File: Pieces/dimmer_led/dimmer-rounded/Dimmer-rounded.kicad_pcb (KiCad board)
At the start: 2 copper layers, 67 x 56 mm, 41 parts, among them J1 Conn_01x02_Female, J2 Conn_01X03, J3 TB_1X2, J4 Conn_01x03_Female, J5 TB_1X2, J6 TB_1X2, Q1 BTA06-600C, Q2 BTA06-600C, Q3 BTA06-600C, Q5 2N7000, U1 LM78XX, U14 LM324, U3 MOC3020M, U4 MOC3020M, U5 MOC3020M, U7 PC817

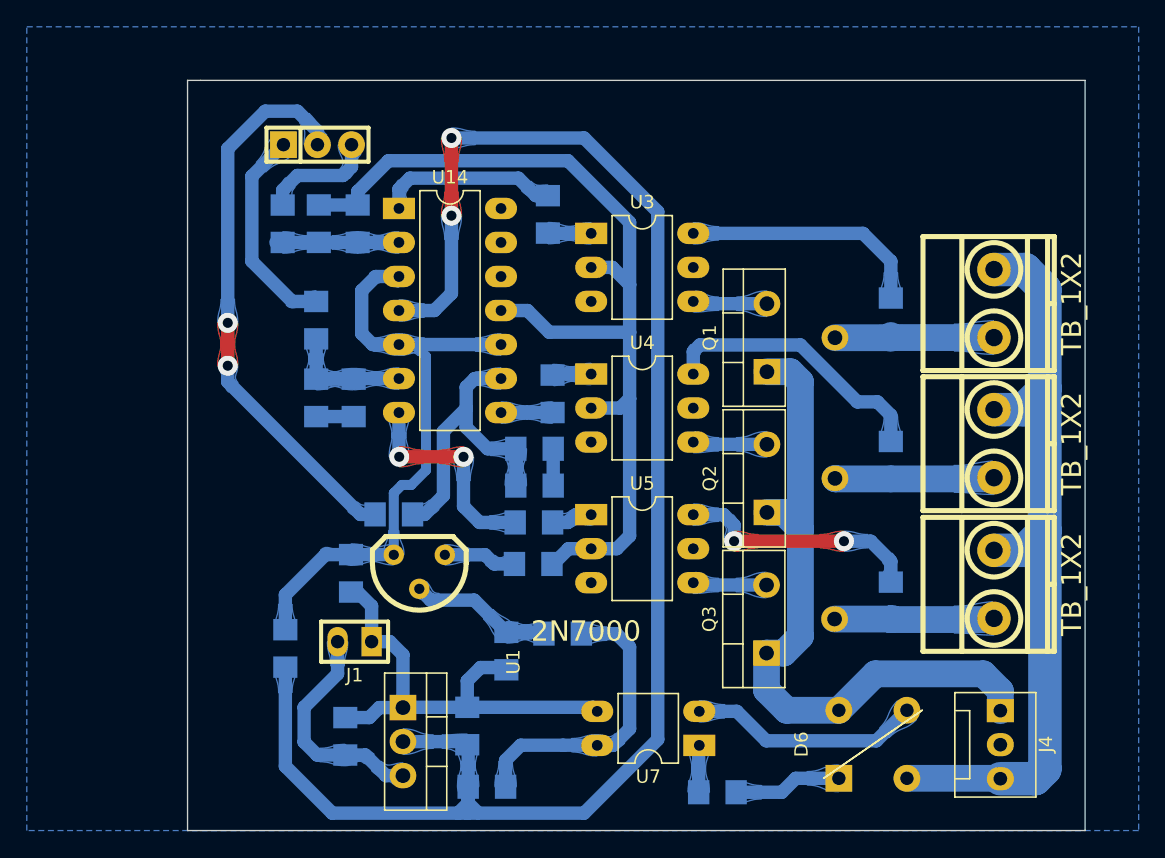
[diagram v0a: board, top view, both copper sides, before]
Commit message: lista de componentes
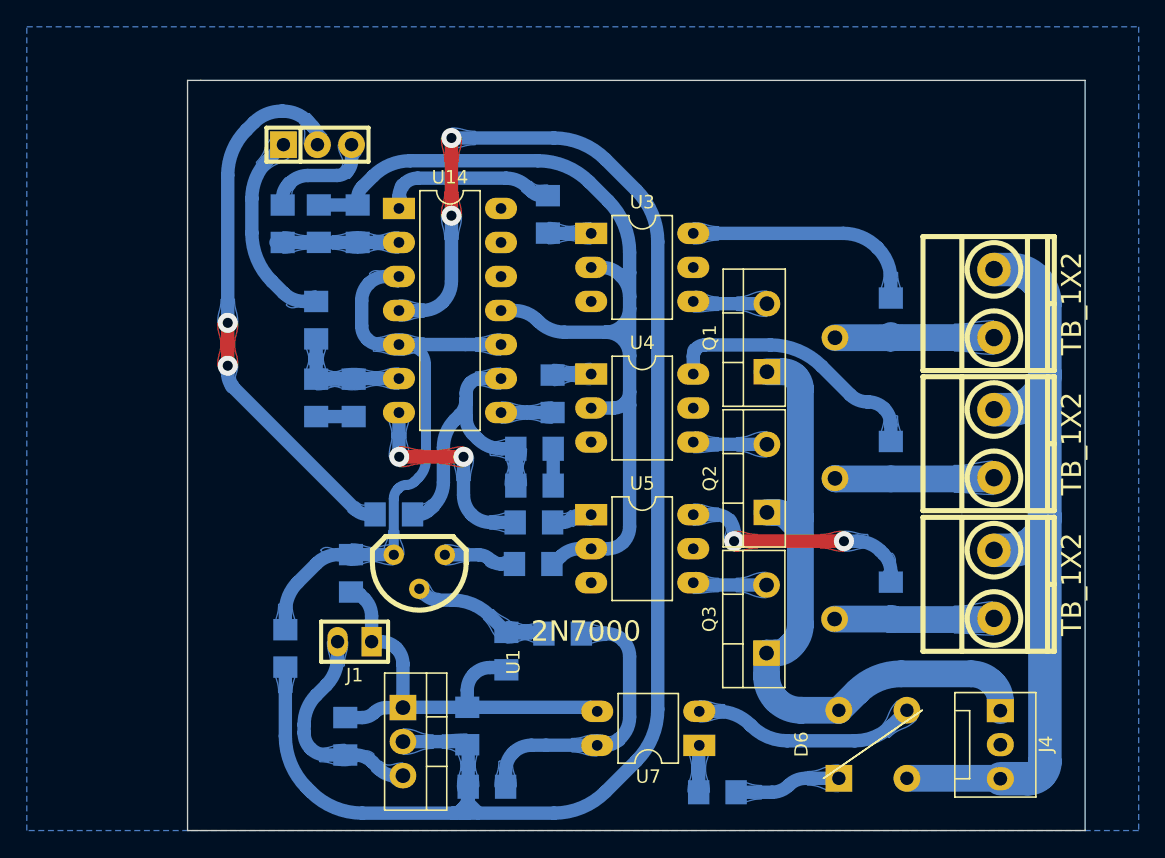
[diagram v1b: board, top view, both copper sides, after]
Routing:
- net GND: track 115.5 -> 119.3 mm
- net Earth: track 59.7 -> 63.0 mm
- net +5V: track 125.8 -> 125.0 mm
- net /Int2: track 42.0 -> 41.3 mm
- net Net-(C23-Pad1): track 23.1 -> 23.7 mm
- net AC: track 51.9 -> 52.4 mm
- net Net-(R25-Pad2): track 21.1 -> 20.6 mm
- net /Int3: track 15.7 -> 15.2 mm
- net Net-(D6-Pad3): track 17.4 -> 16.8 mm
- net Net-(R29-Pad2): track 22.3 -> 21.8 mm
